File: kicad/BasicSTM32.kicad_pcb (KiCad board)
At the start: 4 copper layers, 57.3 x 89.2 mm, 67 parts, among them IC1 TPSM53604RDAR, IC2 LD39100PU33R, J1 1935161, J10 GPIO_OUT PB15, J11 S4B-PH-KL_LF__SN_, J12 TC2050-IDC, J13 USB3131-30-0230-A, J2 Conn_01x01, J3 Conn_01x01, J4 Conn_01x01, J5 Conn_01x02, J6 Conn_01x01, J7 Conn_01x02, J8 DAC1_OUT1, J9 ADC1_IN1, Q1 SI2374DS-T1-GE3, Q2 SI2374DS-T1-GE3, SW1 SW_Push, U1 STM32F303VETx, Y1 NX3225GD-8MHZ-EXS00A-CG04874

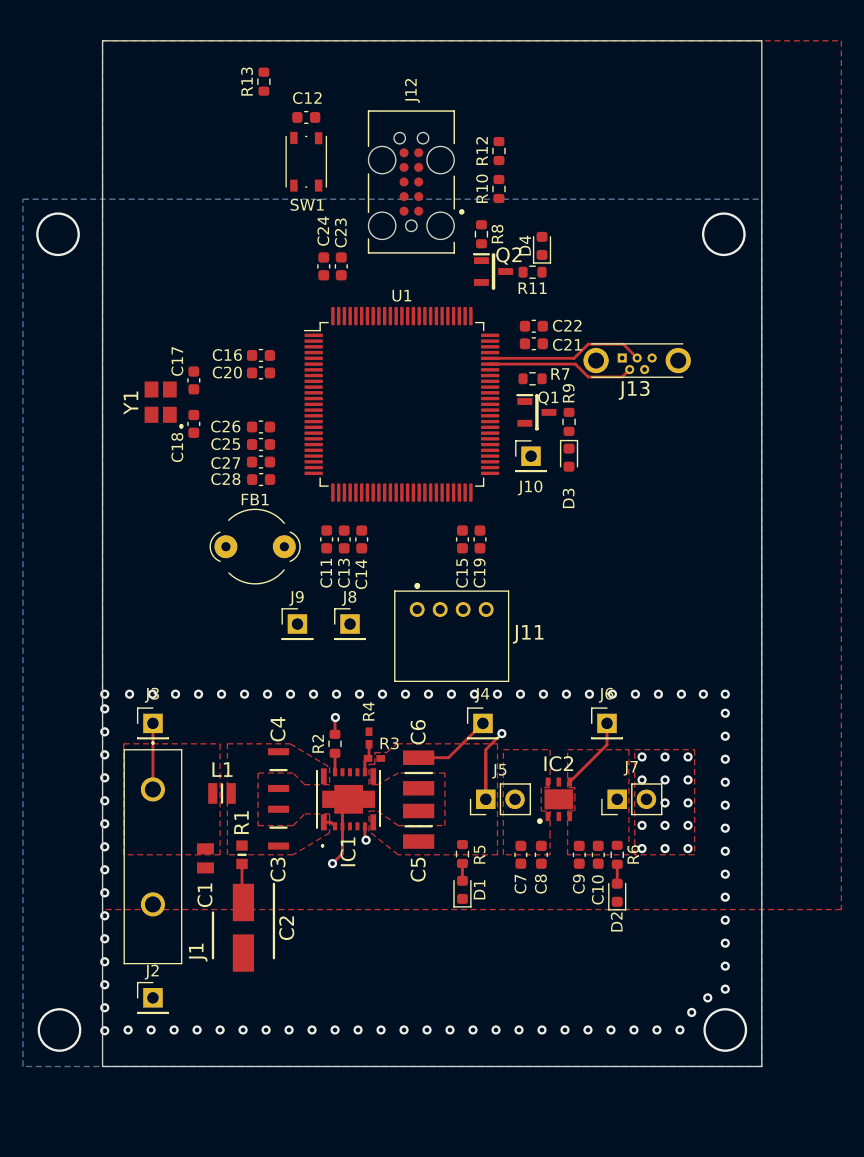
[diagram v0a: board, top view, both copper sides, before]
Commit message: Finish PCB layout and routing
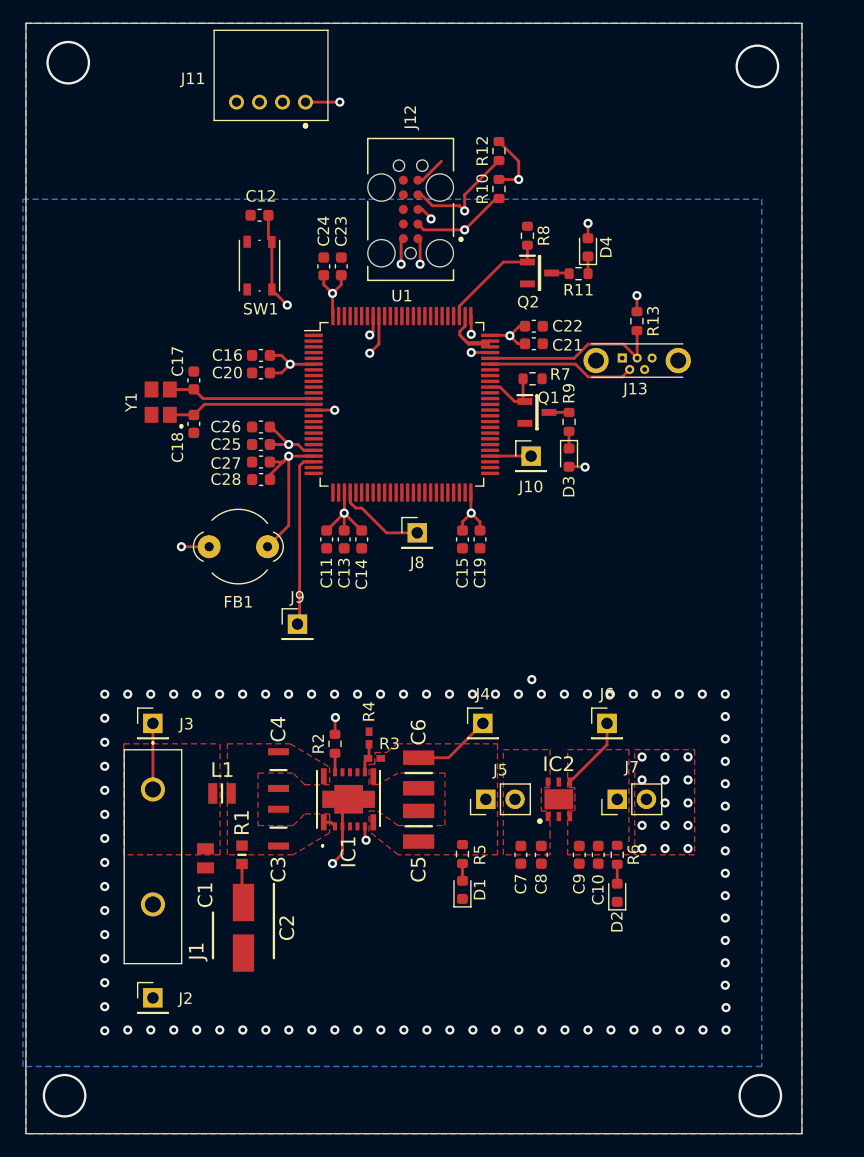
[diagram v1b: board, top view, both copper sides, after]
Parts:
- moved J11 45.2 mm to (83.0, 66.6), turned to 0 degrees
- moved R13 38.6 mm to (111.8, 85.7), turned to 270 degrees
- moved SW1 9.91 mm to (79.0, 80.8)
- moved J8 9.86 mm to (92.7, 104.1)
- moved C12 9.43 mm to (79.0, 76.5)
- moved D4 4.00 mm to (107.6, 79.2)
- moved R11 4.00 mm to (106.7, 81.5)
- moved Q2 4.00 mm to (103.3, 81.5)
- moved R8 4.00 mm to (102.3, 78.2)
- moved J12 2.39 mm to (92.1, 75.9)
- moved FB1 1.46 mm to (74.6, 105.3)
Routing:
- net VDD: track 0.00 -> 50.9 mm, vias 14 -> 26
- net /MCU/NRST: track 0.00 -> 38.6 mm, vias 0 -> 3
- net Net-(J11-Pad2): track 0.00 -> 28.5 mm, vias 0 -> 1
- net Net-(J11-Pad1): track 0.00 -> 26.1 mm, vias 0 -> 2
- net Net-(J12-Pad4): track 0.00 -> 23.7 mm, vias 0 -> 2
- net Net-(J12-Pad2): track 0.00 -> 22.2 mm, vias 0 -> 2
- net /MCU/VDDA22: track 0.00 -> 15.4 mm, vias 0 -> 1
- net Net-(J9-Pad1): track 0.00 -> 15.2 mm
- net +5V: track 58.6 -> 45.3 mm
- net Net-(C18-Pad1): track 0.00 -> 12.9 mm
- net Net-(C17-Pad2): track 0.00 -> 12.8 mm
- net GND: track 6.18 -> 18.5 mm, vias 84 -> 85
- net Net-(Q2-Pad1): track 0.00 -> 9.84 mm
- net Net-(J8-Pad1): track 0.00 -> 7.79 mm
- net Net-(Q1-Pad1): track 0.00 -> 5.57 mm
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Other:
- board size 57.3 x 89.2 mm -> 67.5 x 96.6 mm
